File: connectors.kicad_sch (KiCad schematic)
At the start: 5 parts, among them J1 112-024-113R001, J3 RJHSE5380, J4 USB4085-GF-A

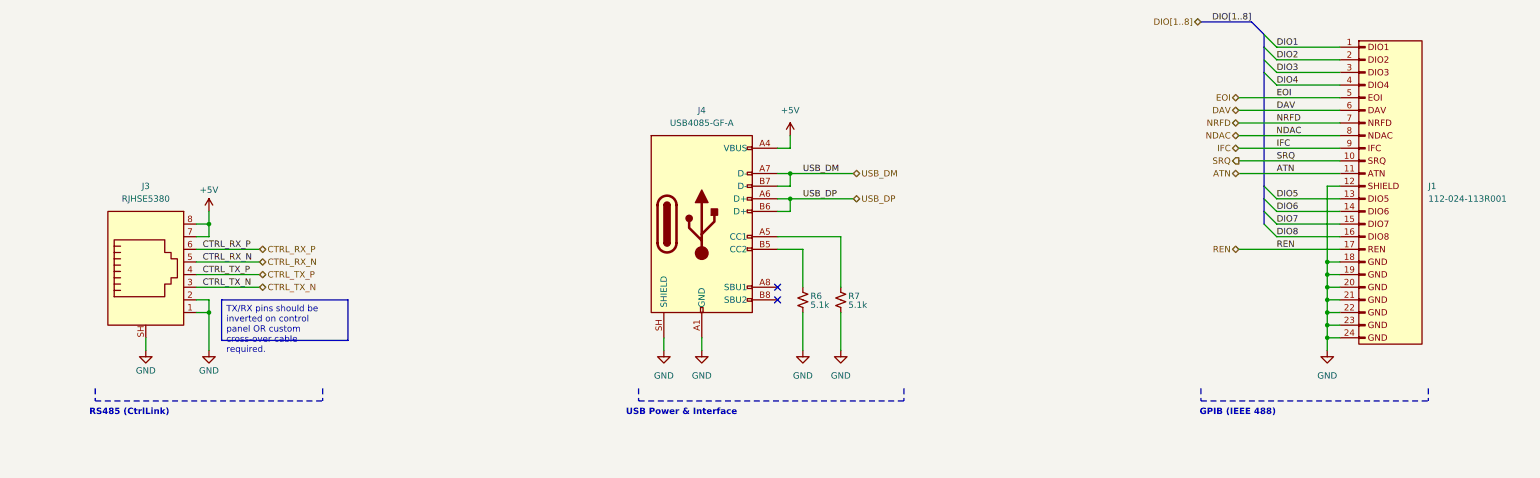
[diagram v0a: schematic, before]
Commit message: Update name
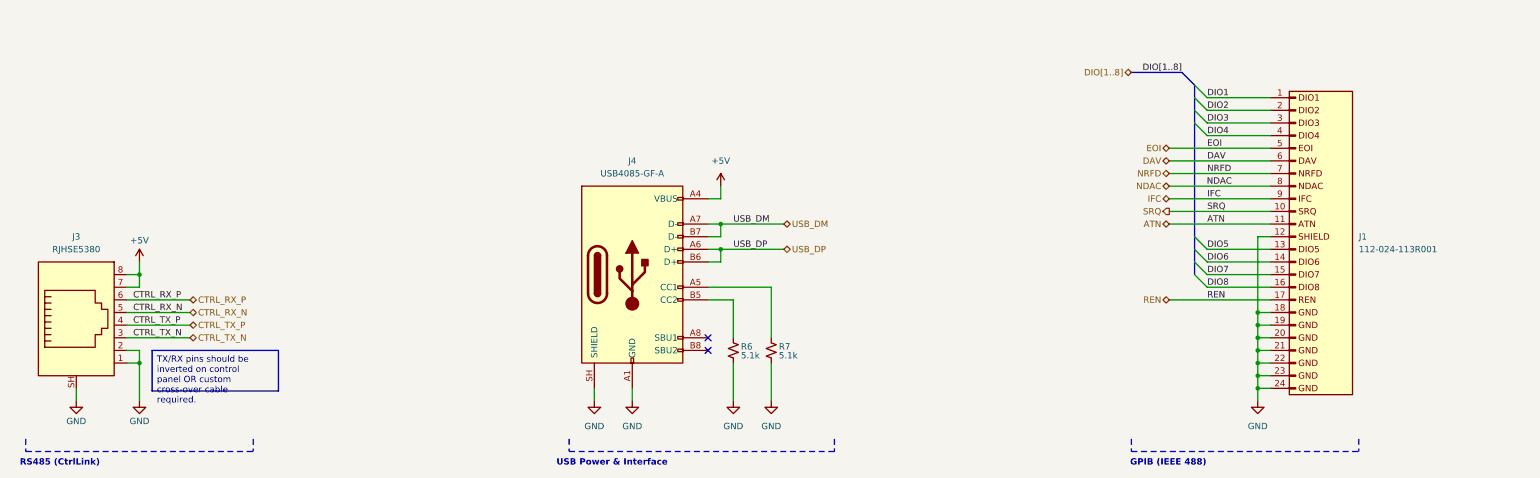
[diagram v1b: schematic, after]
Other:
- moved on the sheet: J1, J3, J4, R6, R7
